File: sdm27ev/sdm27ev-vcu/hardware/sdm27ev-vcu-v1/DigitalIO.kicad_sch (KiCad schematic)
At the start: 28 parts, among them IC17 TPD4E05U06QDQARQ1, IC18 TPD4E05U06QDQARQ1, IC19 TPD4E05U06QDQARQ1, U2 TBD62783AFNG_EL, U8 LM2903BIPWR, U9 LM2903BIPWR

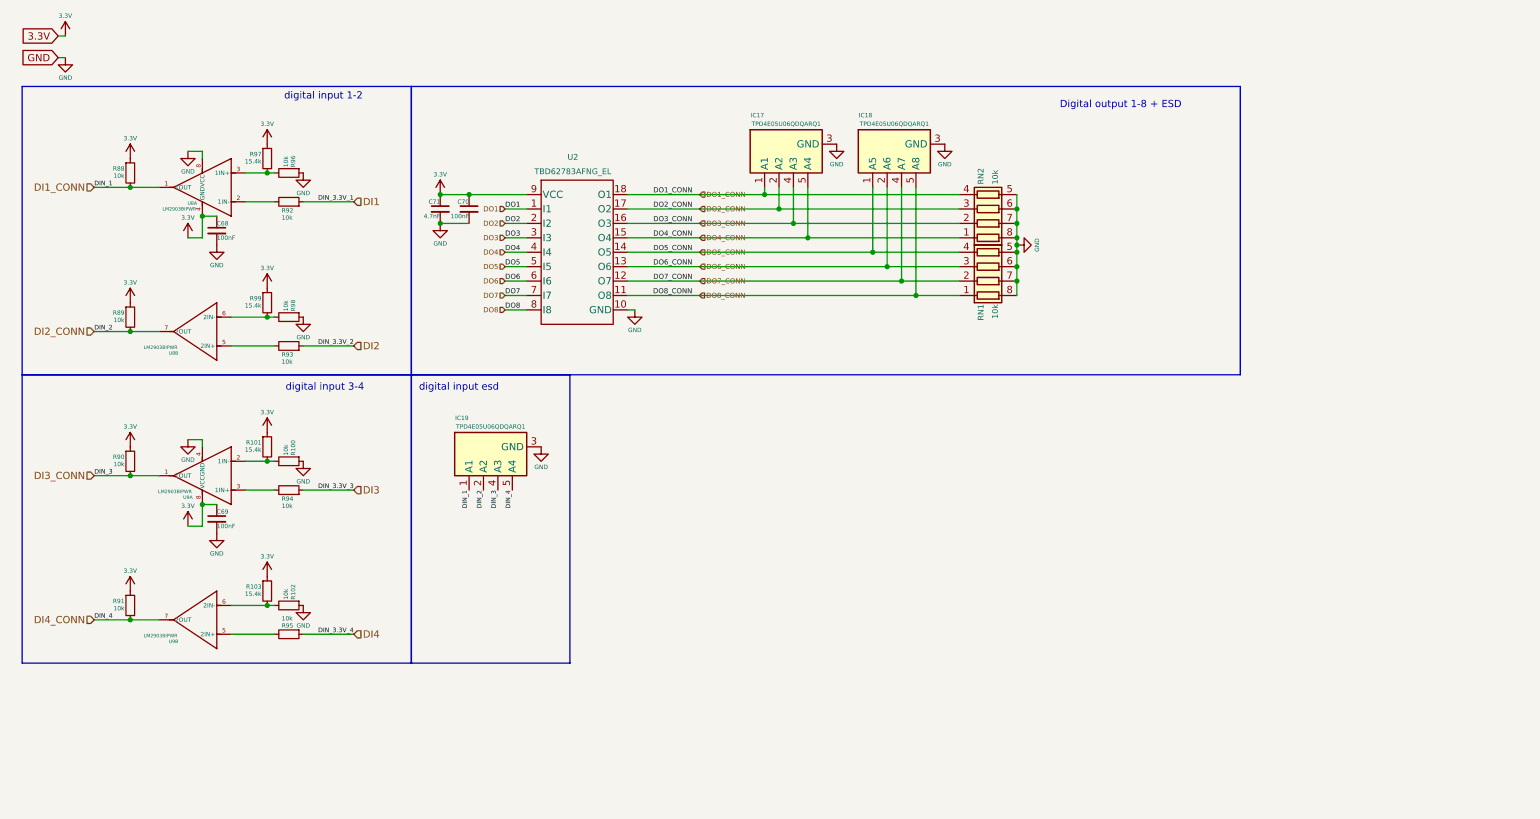
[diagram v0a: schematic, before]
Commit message: VCU updates
Updated P4 Symbol
Digital IO protection rework done
Added pending fixes from design review, e.x SDMC pullups
Needs power review - add this to ToDo
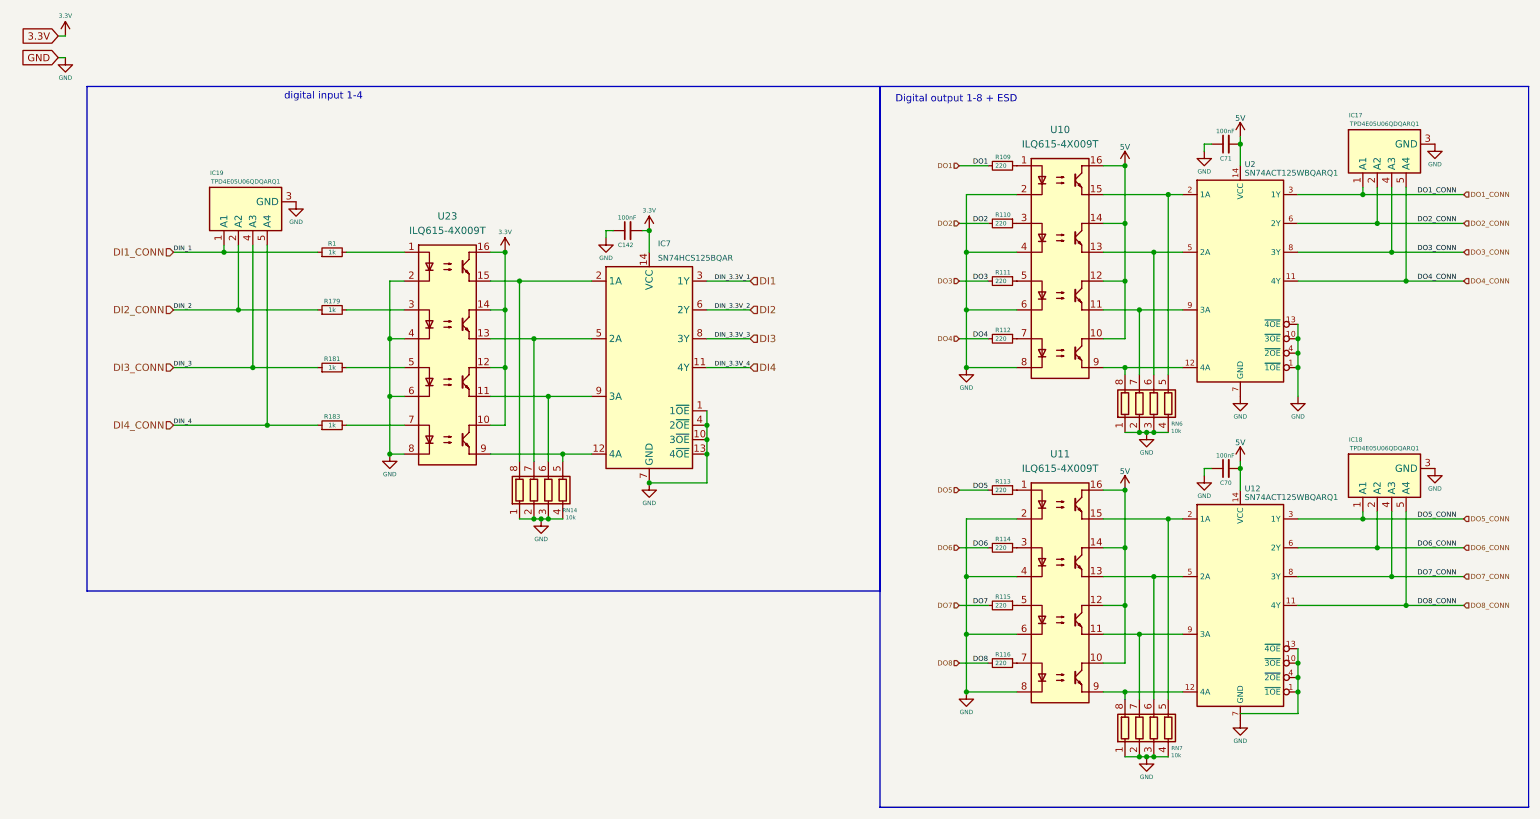
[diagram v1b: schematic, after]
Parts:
- removed C68, C69: 100nF, Capacitor_SMD:C_0603_1608Metric, symbol Device:C_Small
- removed R100, R102, R88, R89, R90, R91, R92, R93, R94, R95, R96, R98: 10k, Resistor_SMD:R_0603_1608Metric, symbol Device:R_Small
- removed R101, R103, R97, R99: 15.4k, Resistor_SMD:R_0603_1608Metric, symbol Device:R_Small
- removed RN1, RN2: 10k, Resistor_SMD:R_Array_Convex_4x0603, symbol Device:R_Pack04
- removed U2: TBD62783AFNG_EL, SSOP18-P-225-0p65_TOS, symbol SDM EV:TBD62783AFNG_EL
- removed U8, U9: LM2903BIPWR, PW0008A-IPC_A, symbol SDM_EV:LM2903BIPWR
- added C142: 100nF, Capacitor_SMD:C_0603_1608Metric, symbol Device:C_Small
- added IC7: SN74HCS125BQAR, SN74HCS125BQAR, symbol SDM_EV:SN74HCS125BQAR
- added R1, R179, R181, R183: 1k, Resistor_SMD:R_0603_1608Metric, symbol Device:R_Small
- added R109, R110, R111, R112, R113, R114, R115, R116: 220, Resistor_SMD:R_0603_1608Metric, symbol Device:R_Small
- added RN14, RN6, RN7: 10k, Resistor_SMD:R_Array_Convex_4x0603, symbol Device:R_Pack04
- added U10, U11, U23: ILQ615-4X009T, SDM_EV:SOIC254P1005X380-16N, symbol SDM_EV:ILQ615-4X009T
- added U12, U2: SN74ACT125WBQARQ1, SN74ACT125_WBQA:SN74ACT125WBQARQ1_WQFN-14-1EP_2.5x3mm_P0.5mm, symbol SDM_EV:SN74ACT125WBQARQ1
- C71: value 4.7nF -> 100nF
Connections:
- net 3.3V: now also C142.2, IC7.14 (VCC), U23.10, U23.12, U23.14, U23.16; no longer C70.1, C71.1
- net DI1: now also IC7.3 (1Y)
- net DI1_CONN: now also R1.1
- net DI2: now also IC7.6 (2Y)
- net DI2_CONN: now also R179.1
- net DI3: now also IC7.8 (3Y)
- net DI3_CONN: now also R181.1
- net DI4: now also IC7.11 (4Y)
- net DI4_CONN: now also R183.1
- net DO1: now also R109.2
- net DO1_CONN: now also U2.3 (1Y)
- net DO2: now also R110.2
- net DO2_CONN: now also U2.6 (2Y)
- net DO3: now also R111.2
- net DO3_CONN: now also U2.8 (3Y)
- net DO4: now also R112.2
- net DO4_CONN: now also U2.11 (4Y)
- net DO5: now also R113.2
- net DO5_CONN: now also U12.3 (1Y)
- net DO6: now also R114.2
- net DO6_CONN: now also U12.6 (2Y)
- net DO7: now also R115.2
- net DO7_CONN: now also U12.8 (3Y)
- net DO8: now also R116.2
- net DO8_CONN: now also U12.11 (4Y)
- net GND: now also C70.1, C71.1, C142.1, IC7.1 (1~{OE}), IC7.10 (3~{OE}), IC7.13 (4~{OE}), IC7.15 (EP), IC7.4 (2~{OE}), IC7.7 (GND), RN14.1 (R1.1), RN14.2 (R2.1), RN14.3 (R3.1), RN14.4 (R4.1), RN6.1 (R1.1), RN6.2 (R2.1), RN6.3 (R3.1), RN6.4 (R4.1), RN7.1 (R1.1), RN7.2 (R2.1), RN7.3 (R3.1), RN7.4 (R4.1), U10.2, U10.4, U10.6, U10.8, U11.2, U11.4, U11.6, U11.8, U12.15 (EP_(GND/NC)), U12.7 (GND), U2.1 (~{1OE}), U2.10 (~{3OE}), U2.13 (~{4OE}), U2.15 (EP_(GND/NC)), U2.4 (~{2OE}), U2.7 (GND), U23.2, U23.4, U23.6, U23.8; no longer C70.2, C71.2
- new net: R112.1, U10.7
- new net: R179.2, U23.3
- new net: U12.1 (~{1OE}), U12.10 (~{3OE}), U12.13 (~{4OE}), U12.4 (~{2OE})
- new net: RN7.8 (R1.2), U11.9, U12.12 (4A)
- new net: RN7.5 (R4.2), U11.15, U12.2 (1A)
- new net: RN7.6 (R3.2), U11.13, U12.5 (2A)
- new net: RN7.7 (R2.2), U11.11, U12.9 (3A)
- new net: R113.1, U11.1
- new net: R114.1, U11.3
- new net: R115.1, U11.5
- new net: R116.1, U11.7
- new net: R1.2, U23.1
- new net: IC7.9 (3A), RN14.6 (R3.2), U23.11
- new net: IC7.5 (2A), RN14.7 (R2.2), U23.13
- new net: IC7.2 (1A), RN14.8 (R1.2), U23.15
- new net: R181.2, U23.5
- new net: R183.2, U23.7
- new net: IC7.12 (4A), RN14.5 (R4.2), U23.9
- new net: R109.1, U10.1
- new net: RN6.7 (R2.2), U10.11, U2.9 (3A)
- new net: RN6.6 (R3.2), U10.13, U2.5 (2A)
- new net: RN6.5 (R4.2), U10.15, U2.2 (1A)
- new net: R110.1, U10.3
- new net: R111.1, U10.5
- new net: RN6.8 (R1.2), U10.9, U2.12 (4A)
- new net 5V: C70.2, C71.2, U10.10, U10.12, U10.14, U10.16, U11.10, U11.12, U11.14, U11.16, U12.14 (VCC), U2.14 (VCC)
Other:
- note added: "digital input 1-4"
- note removed: "digital input 1-2"
- note removed: "digital input 3-4"
- note removed: "digital input esd"
- moved on the sheet: IC17, IC19
